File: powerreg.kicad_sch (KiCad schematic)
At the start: 76 parts, among them J21 USB_C_Receptacle_USB2.0_16P, Q18 SQJ407EP-T1_GE3, Q19 SQJ407EP-T1_GE3, U11 AP22811AW5-7, U3 TPS54531DDAR, U5 TPS54331DR, U6 2920L500/30GR, U8 TPS54331DR

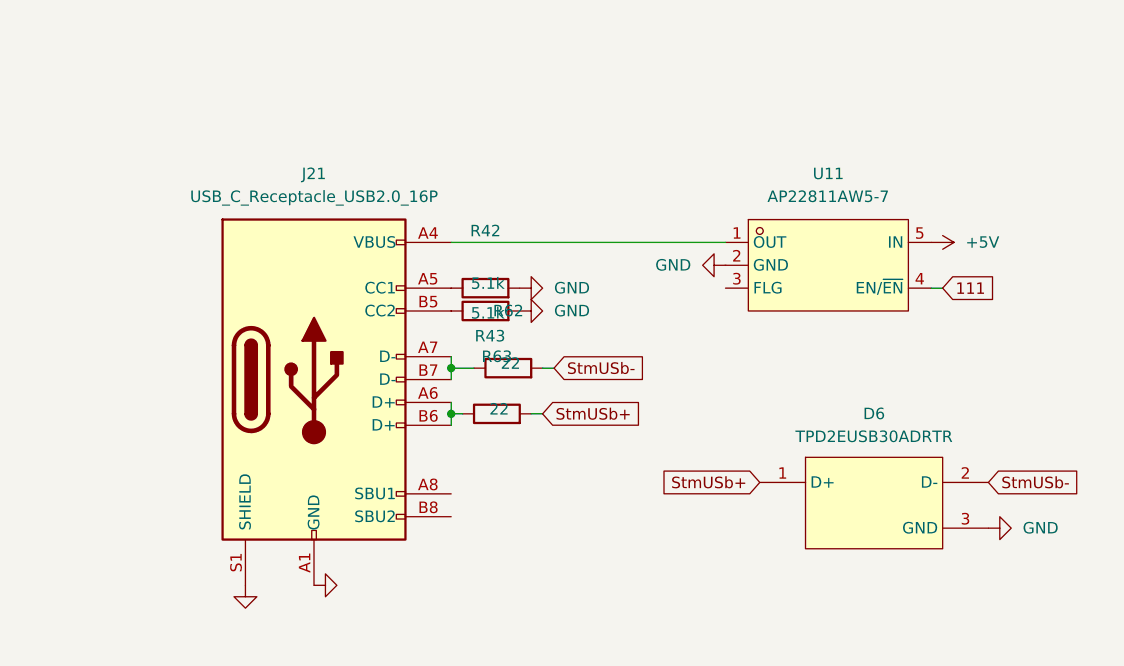
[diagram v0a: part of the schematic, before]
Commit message: Updated schematic and routed PCB
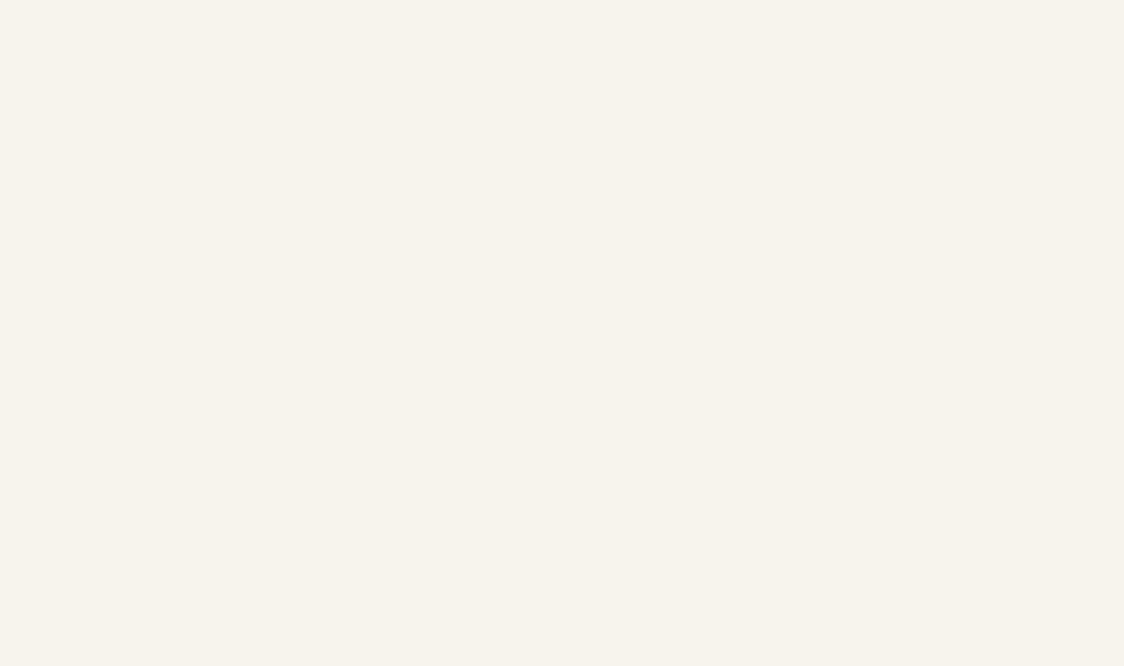
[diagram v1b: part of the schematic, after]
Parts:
- removed D6: TPD2EUSB30ADRTR, easyeda2kicad:SOT-9X3-3_L1.0-W0.8-P0.35-LS1.0-BR, symbol easyeda2kicad:TPD2EUSB30ADRTR
- removed J21: USB_C_Receptacle_USB2.0_16P, Connector_USB:USB_C_Receptacle_HRO_TYPE-C-31-M-12, symbol Connector:USB_C_Receptacle_USB2.0_16P
- removed R42, R43: 5.1k, Resistor_SMD:R_0603_1608Metric, symbol Device:R
- removed R62, R63: 22, Resistor_SMD:R_0603_1608Metric, symbol Device:R
- removed U11: AP22811AW5-7, easyeda2kicad:SOT-25-5_L3.0-W1.6-P0.95-LS2.8-BL, symbol easyeda2kicad:AP22811AW5-7
